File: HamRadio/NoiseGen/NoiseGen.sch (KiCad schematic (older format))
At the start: 20 parts, among them J3 DCJ0202, P1 BNC, Q1 2N3904, Q2 2N3904

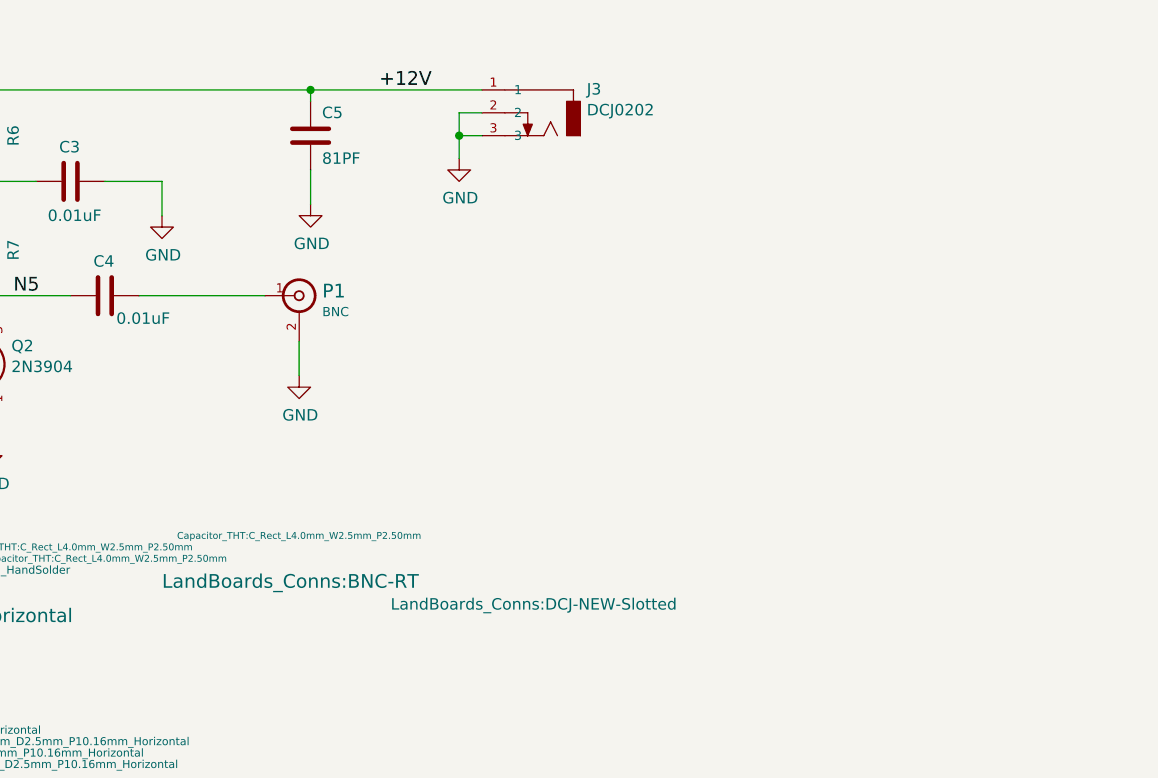
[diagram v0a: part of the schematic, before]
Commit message: FAB NOISE GEN
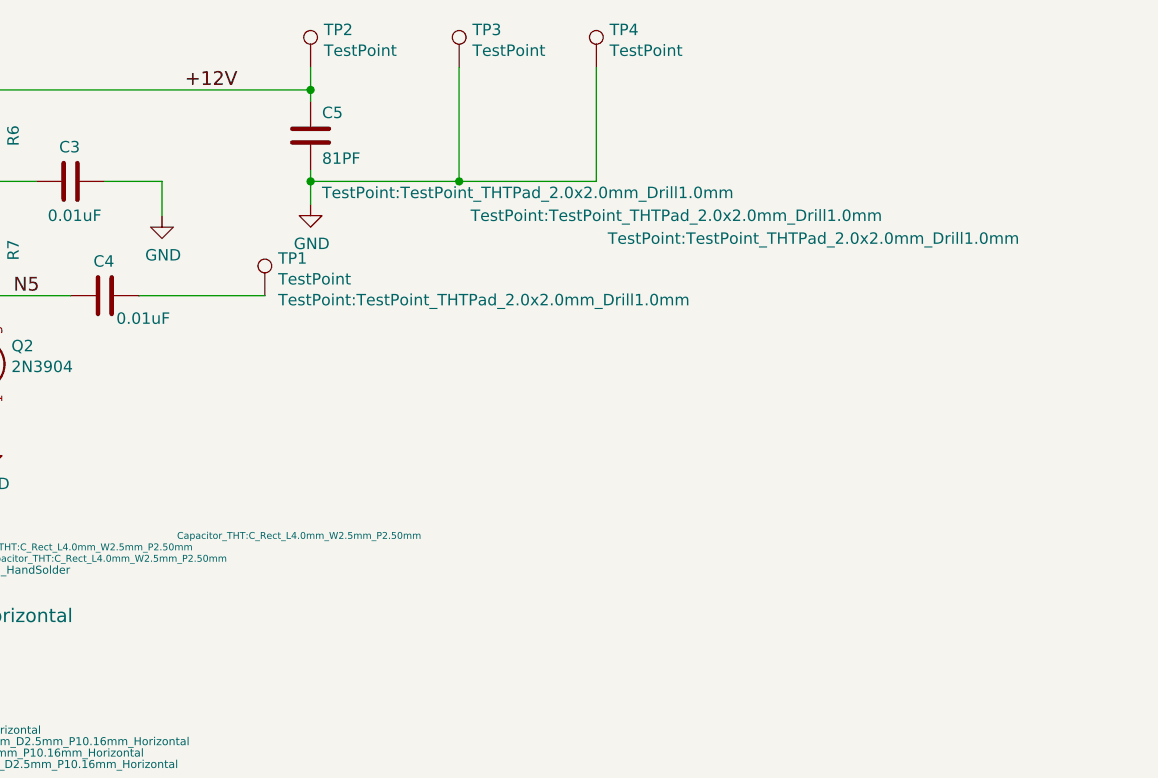
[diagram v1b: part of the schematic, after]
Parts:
- removed J3: DCJ0202, LandBoards_Conns:DCJ-NEW-Slotted, symbol LandBoards_Conns:DCJ0202
- removed P1: BNC, LandBoards_Conns:BNC-RT, symbol LandBoards_Conns:BNC
- added TP1, TP2, TP3, TP4: TestPoint, TestPoint:TestPoint_THTPad_2.0x2.0mm_Drill1.0mm, symbol Connector:TestPoint
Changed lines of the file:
@@
-$EndComp
-$Comp
-L LandBoards_Conns:DCJ0202 J3
-U 1 1 6121F8A4
-P 8000 2900
-F 0 "J3" H 7842 3003 50  0000 R CNN
-F 1 "DCJ0202" H 7842 2912 50  0000 R CNN
-F 2 "LandBoards_Conns:DCJ-NEW-Slotted" H 8700 750 50  0000 R CNN
-F 3 "" H 8000 2900 60  0000 C CNN
-	1    8000 2900
-	-1   0    0    -1
 $EndComp
 $Comp
@@
 Text Label 3200 3550 0    60   ~ 0
 N1
-Text Label 7250 2800 0    60   ~ 0
+Text Label 6400 2800 0    60   ~ 0
 +12V
 $Comp
@@
 Connection ~ 5550 3150
 Connection ~ 4050 2800
-$Comp
-L LandBoards_Conns:BNC P1
-U 1 1 61264FF9
-P 6900 3700
-F 0 "P1" H 7001 3720 60  0000 L CNN
-F 1 "BNC" H 7001 3629 40  0000 L CNN
-F 2 "LandBoards_Conns:BNC-RT" H 6300 2450 60  0000 L CNN
-F 3 "" H 6900 3700 60  0000 C CNN
-	1    6900 3700
-	1    0    0    -1
-$EndComp
-$Comp
-L power:GND #PWR0104
-U 1 1 61265739
-P 6900 4050
-F 0 "#PWR0104" H 6900 3800 50  0001 C CNN
-F 1 "GND" H 6905 3877 50  0000 C CNN
-F 2 "" H 6900 4050 50  0001 C CNN
-F 3 "" H 6900 4050 50  0001 C CNN
-	1    6900 4050
-	1    0    0    -1
-$EndComp
-Wire Wire Line
-	6900 3900 6900 4050
 Connection ~ 5550 3700
 Wire Wire Line
@@
 Text Label 5000 3150 0    60   ~ 0
 N6
-$Comp
-L power:GND #PWR0106
-U 1 1 6128189C
-P 7600 3100
-F 0 "#PWR0106" H 7600 2850 50  0001 C CNN
-F 1 "GND" H 7605 2927 50  0000 C CNN
-F 2 "" H 7600 3100 50  0001 C CNN
-F 3 "" H 7600 3100 50  0001 C CNN
-	1    7600 3100
-	1    0    0    -1
-$EndComp
-Wire Wire Line
-	7600 2900 7600 3000
-Wire Wire Line
-	7600 2900 7700 2900
-Wire Wire Line
-	7600 3000 7700 3000
-Connection ~ 7600 3000
-Wire Wire Line
-	7600 3000 7600 3100
-Wire Wire Line
-	7700 2800 6950 2800
 Connection ~ 5550 2800
 $Comp
@@
 Wire Wire Line
 	6950 2800 6950 2850
-Connection ~ 6950 2800
 Wire Wire Line
 	6950 2800 5550 2800
@@
 $EndComp
 Wire Wire Line
-	6950 3150 6950 3300
+	6950 3150 6950 3200
+$Comp
+L Connector:TestPoint TP1
+U 1 1 6120FAAA
+P 6750 3700
+F 0 "TP1" H 6808 3863 50  0000 L CNN
+F 1 "TestPoint" H 6808 3772 50  0000 L CNN
+F 2 "TestPoint:TestPoint_THTPad_2.0x2.0mm_Drill1.0mm" H 6808 3681 50  0000 L CNN
+F 3 "~" H 6950 3700 50  0001 C CNN
+	1    6750 3700
+	1    0    0    -1
+$EndComp
+$Comp
+L Connector:TestPoint TP2
+U 1 1 6120FEFA
+P 6950 2700
+F 0 "TP2" H 7008 2863 50  0000 L CNN
+F 1 "TestPoint" H 7008 2772 50  0000 L CNN
+F 2 "TestPoint:TestPoint_THTPad_2.0x2.0mm_Drill1.0mm" H 7000 2150 50  0000 L CNN
+F 3 "~" H 7150 2700 50  0001 C CNN
+	1    6950 2700
+	1    0    0    -1
+$EndComp
+Wire Wire Line
+	6950 2700 6950 2800
+Connection ~ 6950 2800
+$Comp
+L Connector:TestPoint TP3
+U 1 1 612121CD
+P 7600 2700
+F 0 "TP3" H 7658 2863 50  0000 L CNN
+F 1 "TestPoint" H 7658 2772 50  0000 L CNN
+F 2 "TestPoint:TestPoint_THTPad_2.0x2.0mm_Drill1.0mm" H 7650 2050 50  0000 L CNN
+F 3 "~" H 7800 2700 50  0001 C CNN
+	1    7600 2700
+	1    0    0    -1
+$EndComp
+$Comp
+L Connector:TestPoint TP4
+U 1 1 612138D7
+P 8200 2700
+F 0 "TP4" H 8258 2863 50  0000 L CNN
+F 1 "TestPoint" H 8258 2772 50  0000 L CNN
+F 2 "TestPoint:TestPoint_THTPad_2.0x2.0mm_Drill1.0mm" H 8250 1950 50  0000 L CNN
+F 3 "~" H 8400 2700 50  0001 C CNN
+	1    8200 2700
+	1    0    0    -1
+$EndComp
+Wire Wire Line
+	6950 3200 7600 3200
+Wire Wire Line
+	8200 3200 8200 2700
+Connection ~ 6950 3200
+Wire Wire Line
+	6950 3200 6950 3300
+Wire Wire Line
+	7600 2700 7600 3200
+Connection ~ 7600 3200
+Wire Wire Line
+	7600 3200 8200 3200
 $EndSCHEMATC
